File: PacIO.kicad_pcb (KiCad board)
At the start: 2 copper layers, 68 x 52 mm, 21 parts, among them J1 Conn_01x02_Female, J2 Conn_01x02_Female, J3 Conn_01x08_Male, J4 Conn_01x20_Male

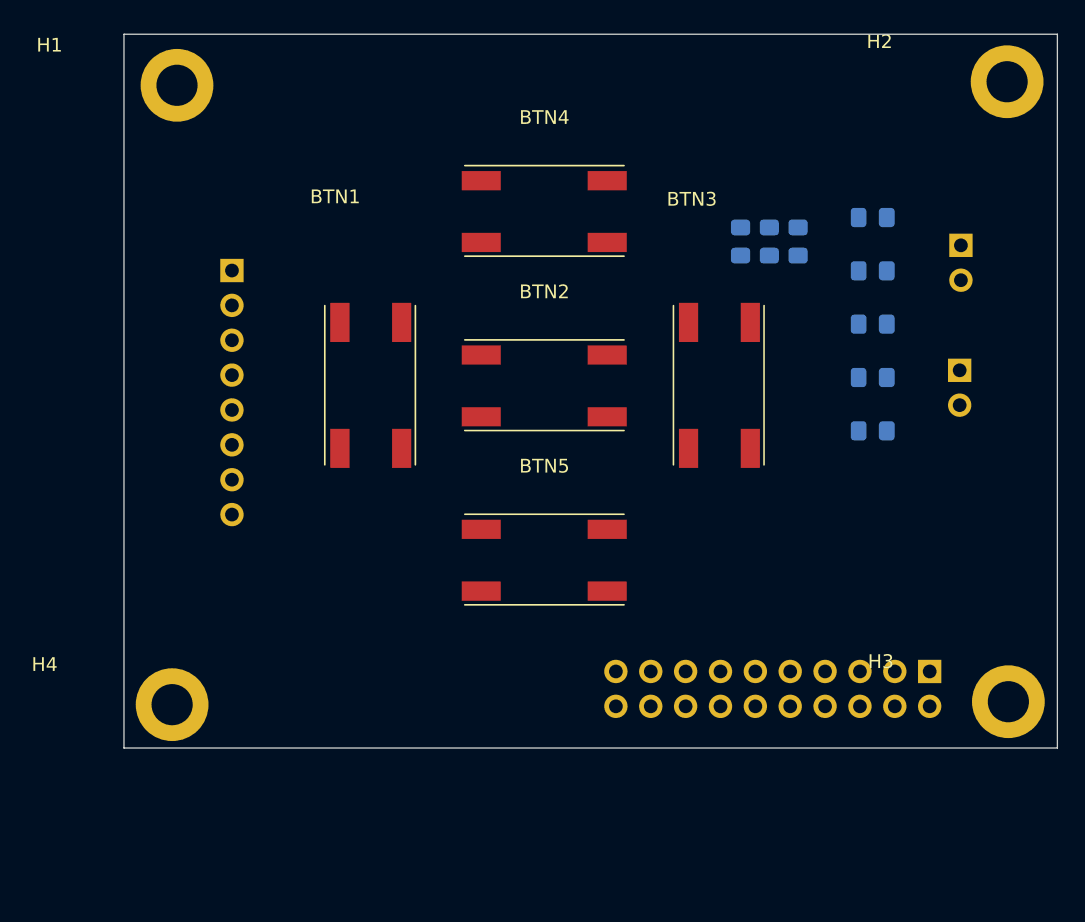
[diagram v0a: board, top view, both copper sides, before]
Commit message: layout
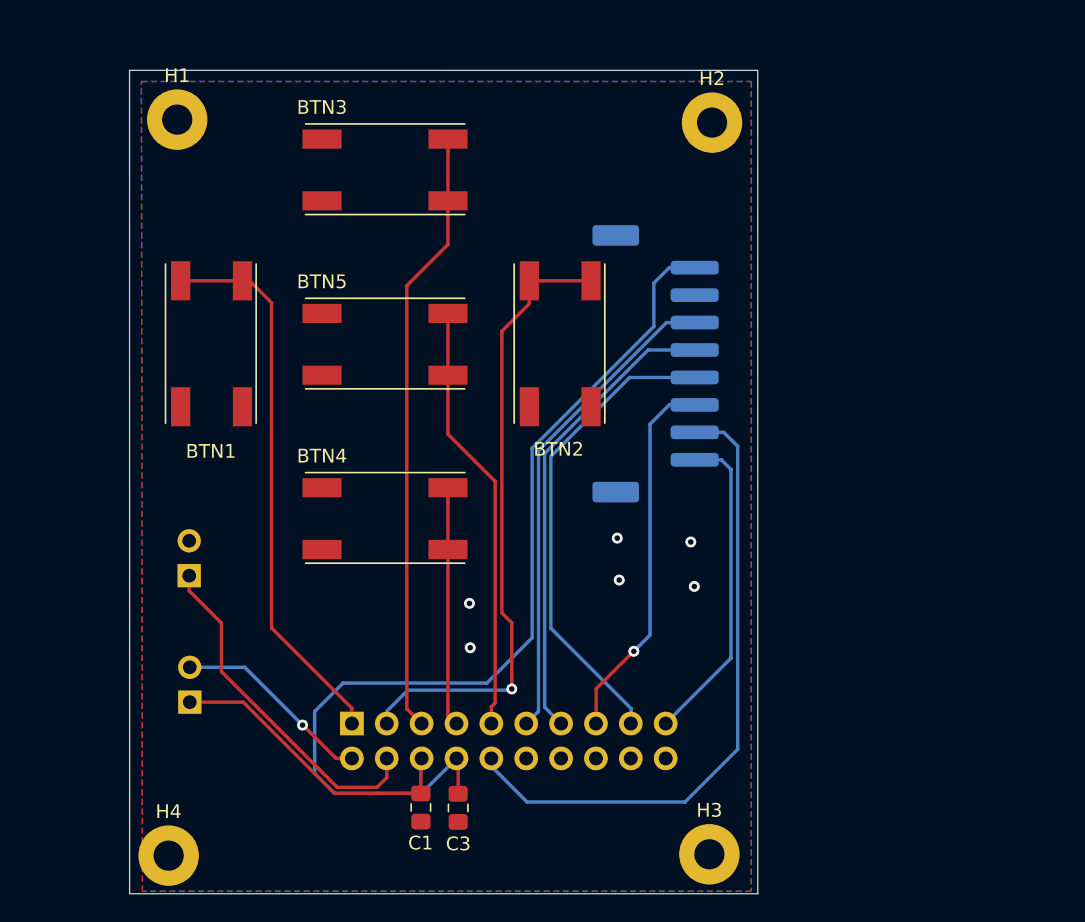
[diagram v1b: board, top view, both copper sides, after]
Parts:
- removed C2: C, Capacitor_SMD:C_0805_2012Metric_Pad1.15x1.40mm_HandSolder
- removed R1, R2, R3, R4, R5: R, Resistor_SMD:R_0805_2012Metric_Pad1.15x1.40mm_HandSolder
- added LOGO1: LafECEDepLogo, Lafayette_Electric_Car_Footprints:ECE_Logo_Jon, B.Cu at (127.5, 114.6)
- added LOGO2: LeopardPawLogo, Lafayette_Electric_Car_Footprints:Paw, B.Cu at (148.6, 130.3)
- BTN2: value PushButton -> BTN_RIGHT
- BTN3: value PushButton -> BTN_UP
- BTN4: value PushButton -> BTN_DOWN
- BTN5: value PushButton -> BTN_CENTER
- C1, C3: moved to F.Cu
- H1, H2, H3, H4: value standoff_smt_M2_3.5mm -> MountingHole_Pad; footprint Lafayette_Electric_Car_Footprints:standoff_smt_m2_3.5mm -> MountingHole:MountingHole_2.2mm_M2_Pad
- J1: value Conn_01x02_Female -> PacMan_Connector; footprint Connector_PinSocket_2.54mm:PinSocket_1x02_P2.54mm_Vertical -> Connector_IDC:IDC-Header_2x10_P2.54mm_Vertical
- J2: value Conn_01x02_Female -> E-ink Display; footprint Connector_PinSocket_2.54mm:PinSocket_1x02_P2.54mm_Vertical -> Connector_JST:JST_PH_S8B-PH-SM4-TB_1x08-1MP_P2.00mm_Horizontal
- J3: value Conn_01x08_Male -> High_Voltage_Indicator; footprint Connector_PinSocket_2.54mm:PinSocket_1x08_P2.54mm_Vertical -> Connector_PinSocket_2.54mm:PinSocket_1x02_P2.54mm_Vertical
- J4: value Conn_01x20_Male -> Charge_Indicator; footprint Connector_PinSocket_2.54mm:PinSocket_2x10_P2.54mm_Vertical -> Connector_PinSocket_2.54mm:PinSocket_1x02_P2.54mm_Vertical
- moved J1 56.4 mm to (126.6, 140.2), turned to 270 degrees
- moved J4 54.0 mm to (114.8, 138.7), turned to 0 degrees
- moved C1 47.4 mm to (131.6, 146.3)
- moved C3 47.1 mm to (134.3, 146.4)
- moved BTN3 29.0 mm to (129.0, 99.8), turned to 0 degrees
- moved BTN4 25.2 mm to (129.0, 125.2)
- moved H3 24.4 mm to (152.6, 149.7)
- moved J3 22.4 mm to (114.8, 129.4), turned to 0 degrees
- moved J2 22.2 mm to (148.7, 114.0), turned to 90 degrees
- moved H2 21.6 mm to (152.8, 96.4)
- moved BTN5 19.5 mm to (129.0, 112.5)
- moved BTN1 12.0 mm to (116.3, 112.5)
- moved H4 11.1 mm to (113.3, 149.8)
- moved BTN2 3.23 mm to (141.7, 112.5), turned to 90 degrees
- moved H1 2.57 mm to (113.9, 96.2)
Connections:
- BTN1 pad 1: /btn_left -> GND
- BTN1 pad 2: +3V3 -> /BTN_LEFT
- BTN2 pad 1: /btn_center -> GND
- BTN2 pad 2: +3V3 -> /BTN_RIGHT
- BTN3 pad 1: /btn_right -> GND
- BTN3 pad 2: +3V3 -> /BTN_UP
- BTN4 pad 1: /btn_up -> GND
- BTN4 pad 2: +3V3 -> /BTN_DOWN
- BTN5 pad 1: /btn_down -> GND
- BTN5 pad 2: +3V3 -> /BTN_CENTER
- C1 pad 1: /indicator1 -> +24V
- H1 pad 1: (no net) -> GND
- H2 pad 1: (no net) -> GND
- H3 pad 1: (no net) -> GND
- H4 pad 1: (no net) -> GND
- J1 pad 1: /indicator1 -> /BTN_LEFT
- J1 pad 2: GND -> /CHRGE_LED
- J2 pad 1: /indicator2 -> /DISP_BUSY
- J2 pad 2: GND -> /DISP_RST
- J3 pad 1: /Busy -> /TSV_LIVE
- J3 pad 2: /RST -> GND
- J4 pad 1: +3V3 -> +24V
- J4 pad 2: /btn_left -> /CHRGE_LED
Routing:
- net +3V3: track 0.00 -> 70.2 mm
- net /DISP_RST: track 0.00 -> 46.8 mm
- net /BTN_RIGHT: track 0.00 -> 46.0 mm, vias 0 -> 1
- net /BTN_UP: track 0.00 -> 44.3 mm
- net /BTN_LEFT: track 0.00 -> 40.4 mm
- net /DISP_DIN: track 0.00 -> 35.5 mm
- net /DISP_CS: track 0.00 -> 34.8 mm
- net /DISP_CLK: track 0.00 -> 34.2 mm
- net /BTN_CENTER: track 0.00 -> 31.4 mm
- net /DISP_DC: track 0.00 -> 27.3 mm, vias 0 -> 1
- net /TSV_LIVE: track 0.00 -> 25.2 mm
- net /DISP_BUSY: track 0.00 -> 24.1 mm
- net +24V: track 0.00 -> 22.2 mm
- net /BTN_DOWN: track 0.00 -> 17.4 mm
- net /CHRGE_LED: track 0.00 -> 14.6 mm, vias 0 -> 1
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- added copper zone on B.Cu, net GND
- added copper zone on F.Cu, net GND
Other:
- board size 68 x 52 mm -> 45.8 x 60 mm
